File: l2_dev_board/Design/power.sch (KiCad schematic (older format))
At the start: 49 parts, among them U1001 LT3480, U1002 NCP1529, U1003 NCP1529, U1004 NCP1529, U1005 APX803-SR, U1006 NCP1529, U1007 NCP1529, U1008 APX803-SR

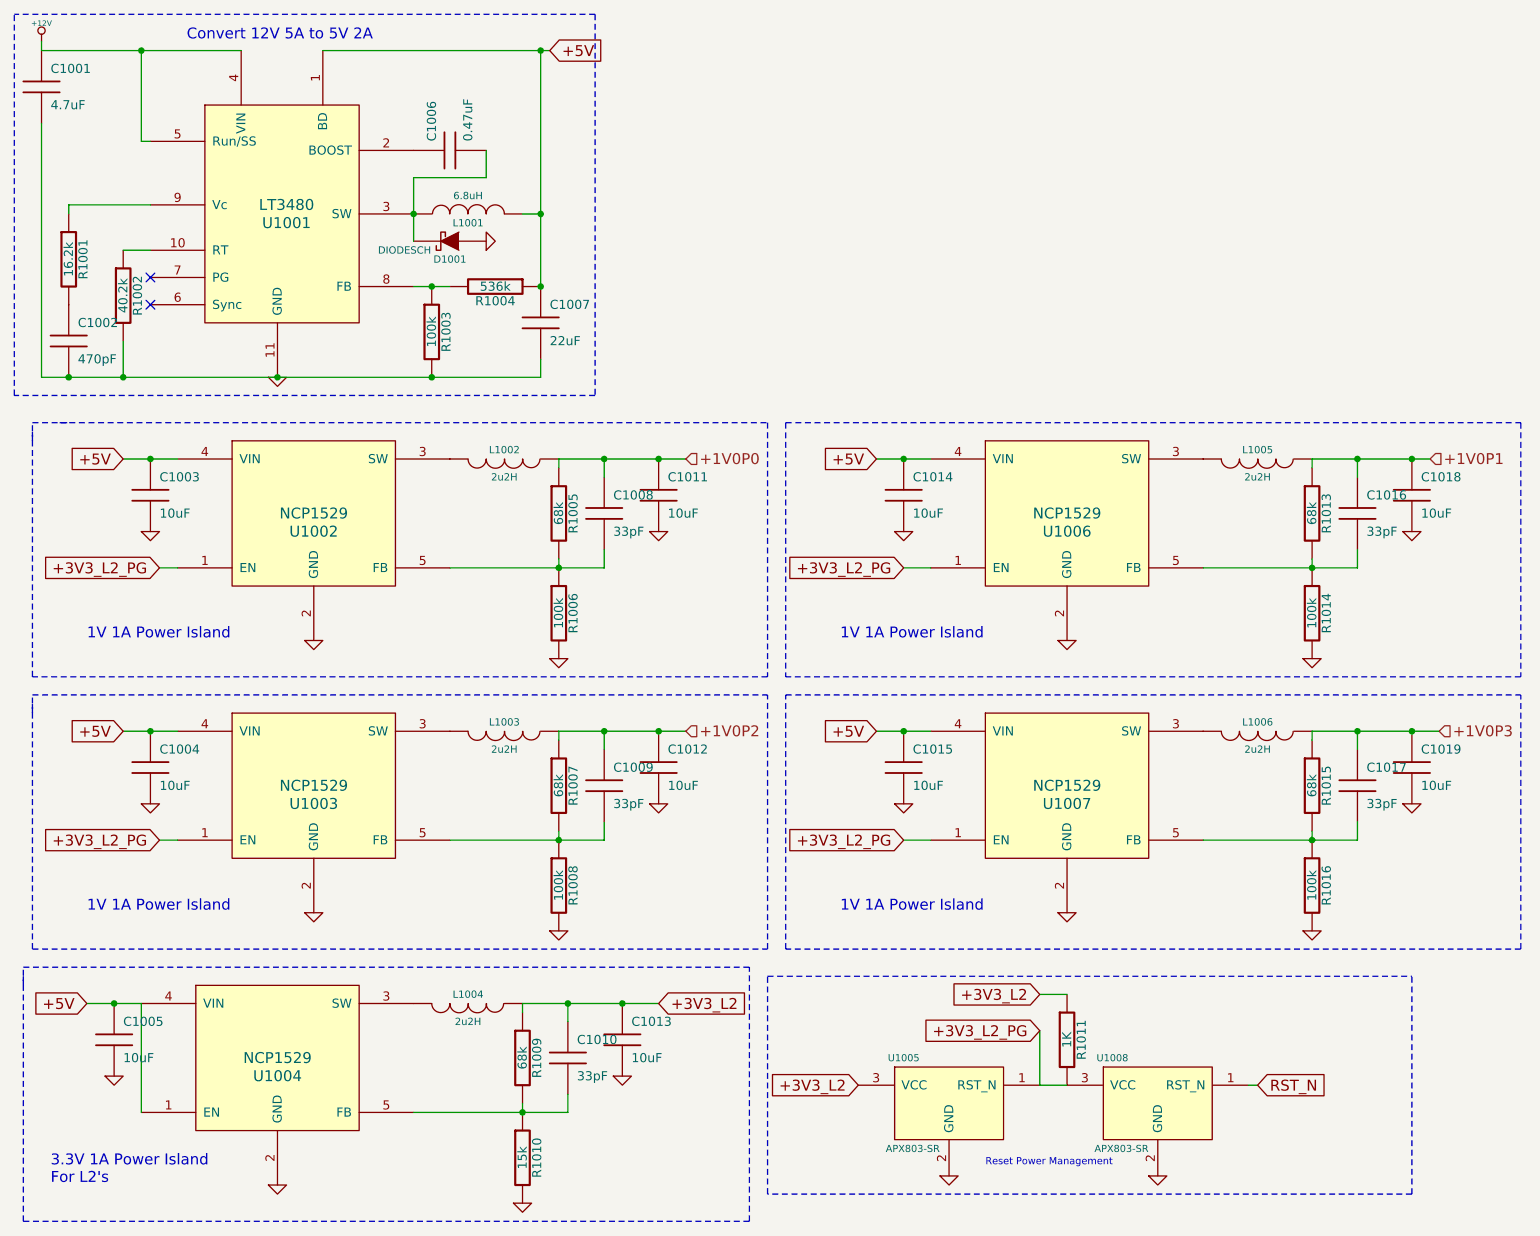
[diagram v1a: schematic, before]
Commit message: missing header connector for 2 L2s. Find space!
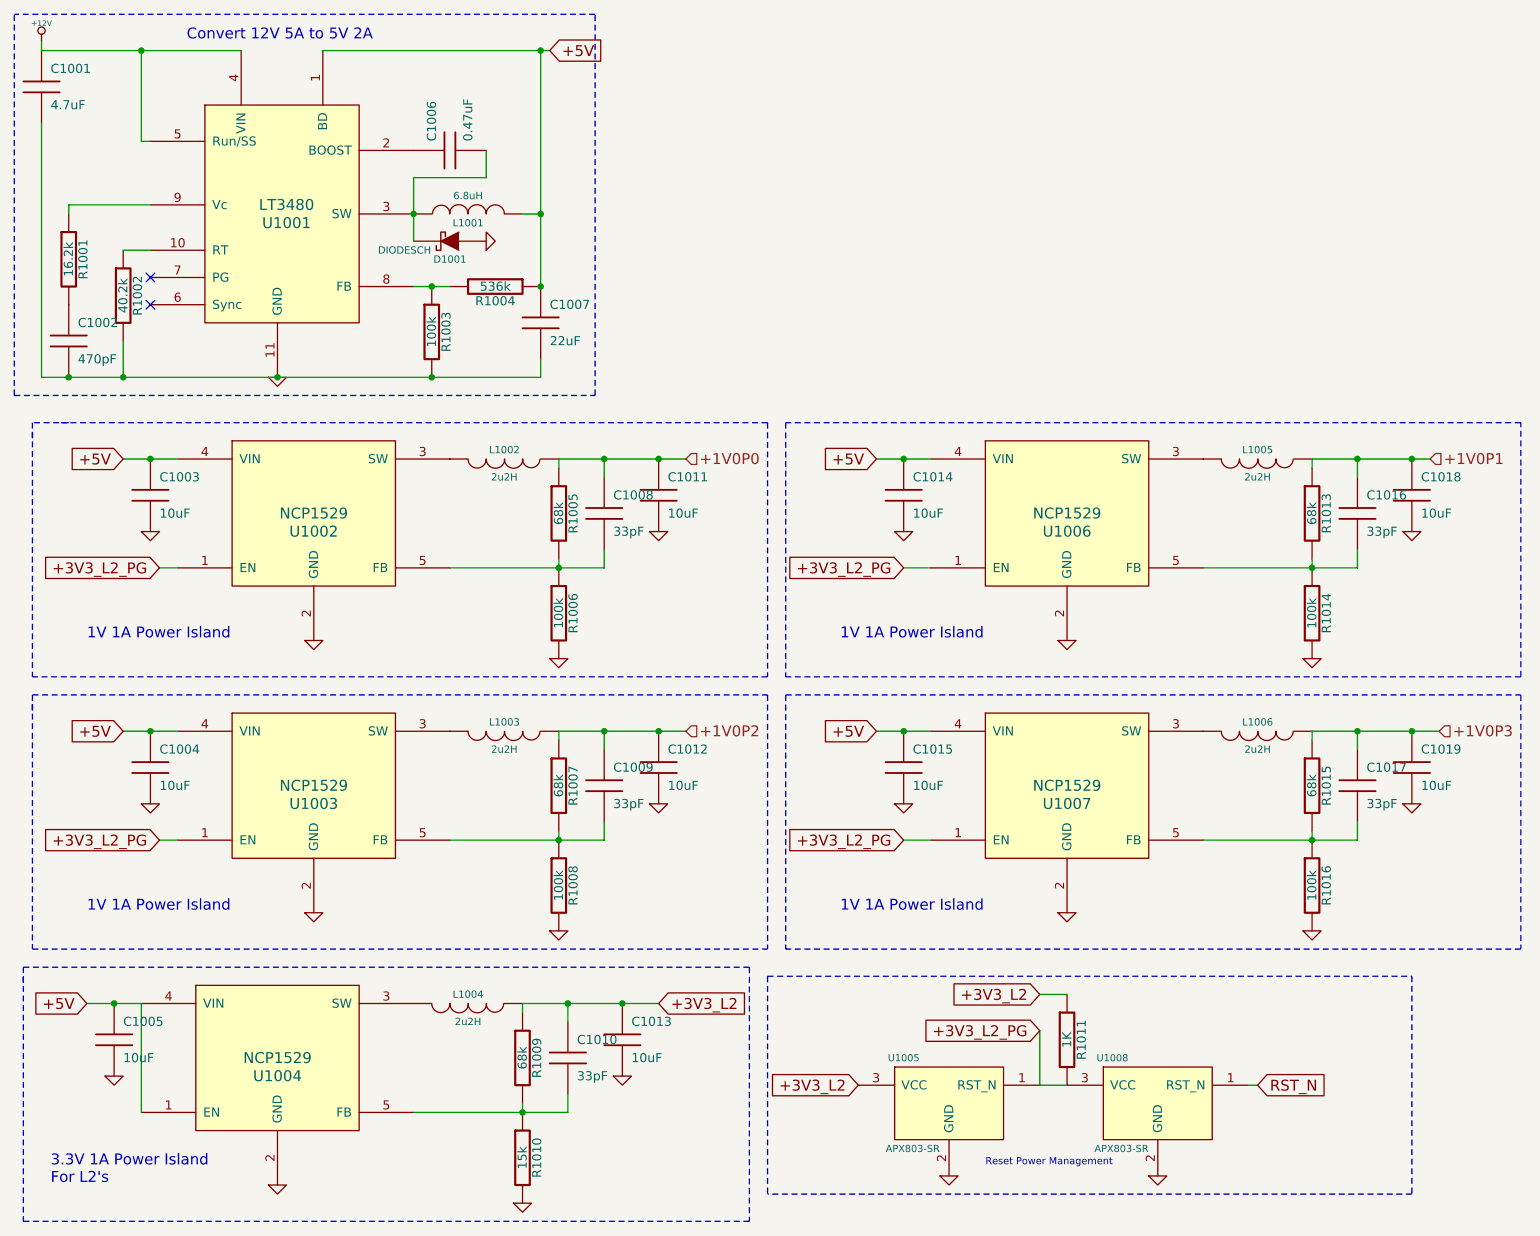
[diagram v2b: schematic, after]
